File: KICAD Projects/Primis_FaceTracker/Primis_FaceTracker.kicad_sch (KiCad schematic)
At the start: 47 parts, among them CN2 KH-FG0.5-H2.0-24PIN, J1 USB_C_Receptacle_USB2.0_16P, Q1 PMOS, SW1 SW_SPST, SW2 SW_SPST, U1 ESP32-S3-WROOM-1, U2 AMS1117-3.3, U3 XC6206P122MR, U5 XC6206P282MR

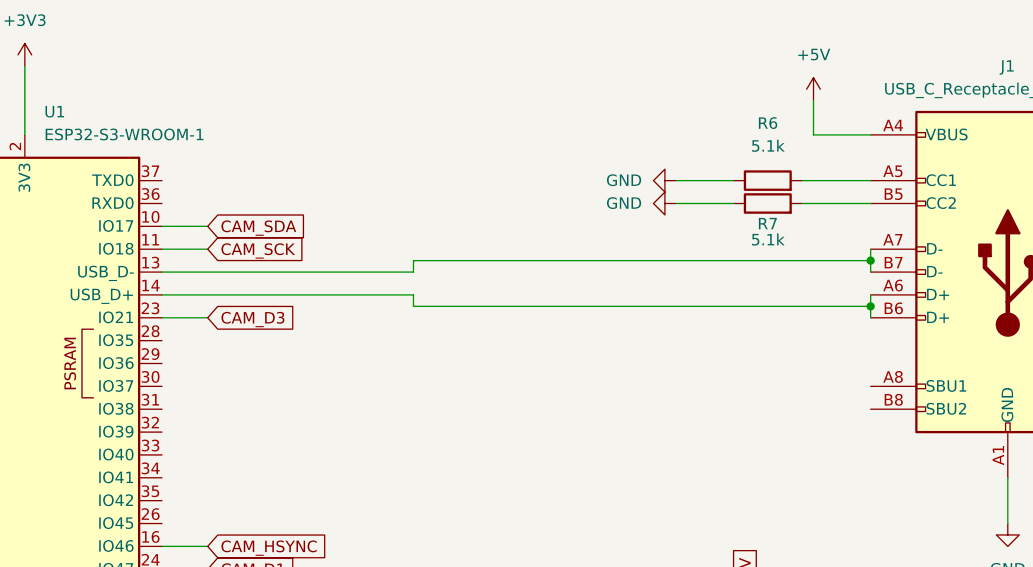
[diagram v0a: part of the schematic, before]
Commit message: Face Tracker PCB
-Some work on the PCB, not quite done but I'm making some changes so uploading as a backup.
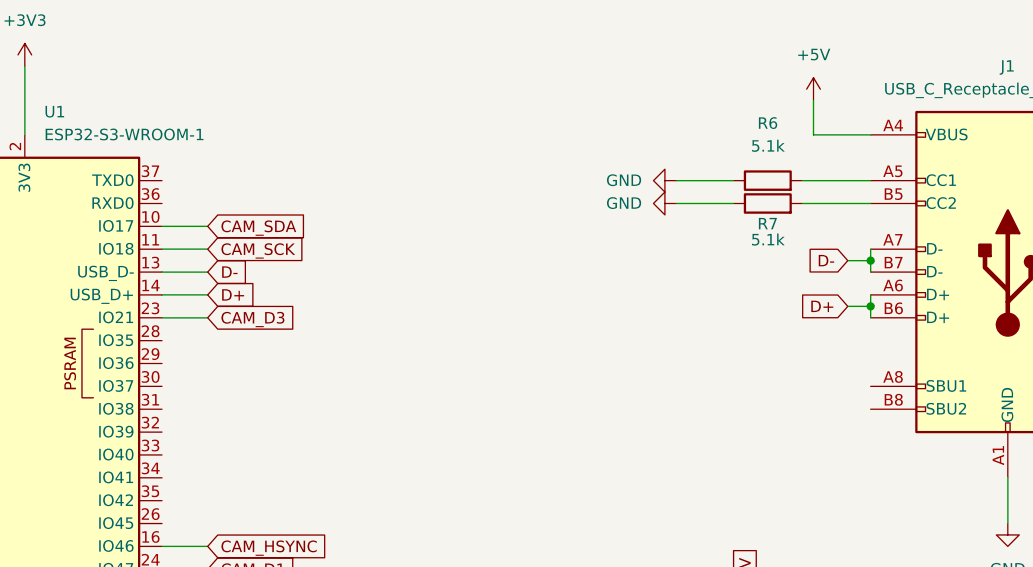
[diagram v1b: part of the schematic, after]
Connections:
- net D-: now reaches J1.A7 (D-), J1.B7 (D-), U1.13 (USB_D-)
- net D+: now reaches J1.A6 (D+), J1.B6 (D+), U1.14 (USB_D+)
